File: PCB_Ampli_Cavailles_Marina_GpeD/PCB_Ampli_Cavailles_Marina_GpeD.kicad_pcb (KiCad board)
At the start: 2 copper layers, 52 parts, among them J2 Conn_01x02, J3 Conn_01x03, Q1 2N2907, Q10 TIP32, Q11 BD138, Q12 TIP31, Q13 2N2222, Q2 2N2907, Q3 2N2907, Q4 2N2222, Q5 2N2222, Q6 2N2907, Q7 2N2907, Q8 BD139, Q9 BD139, U1 Relay_1CT, U2 Jack_Mono

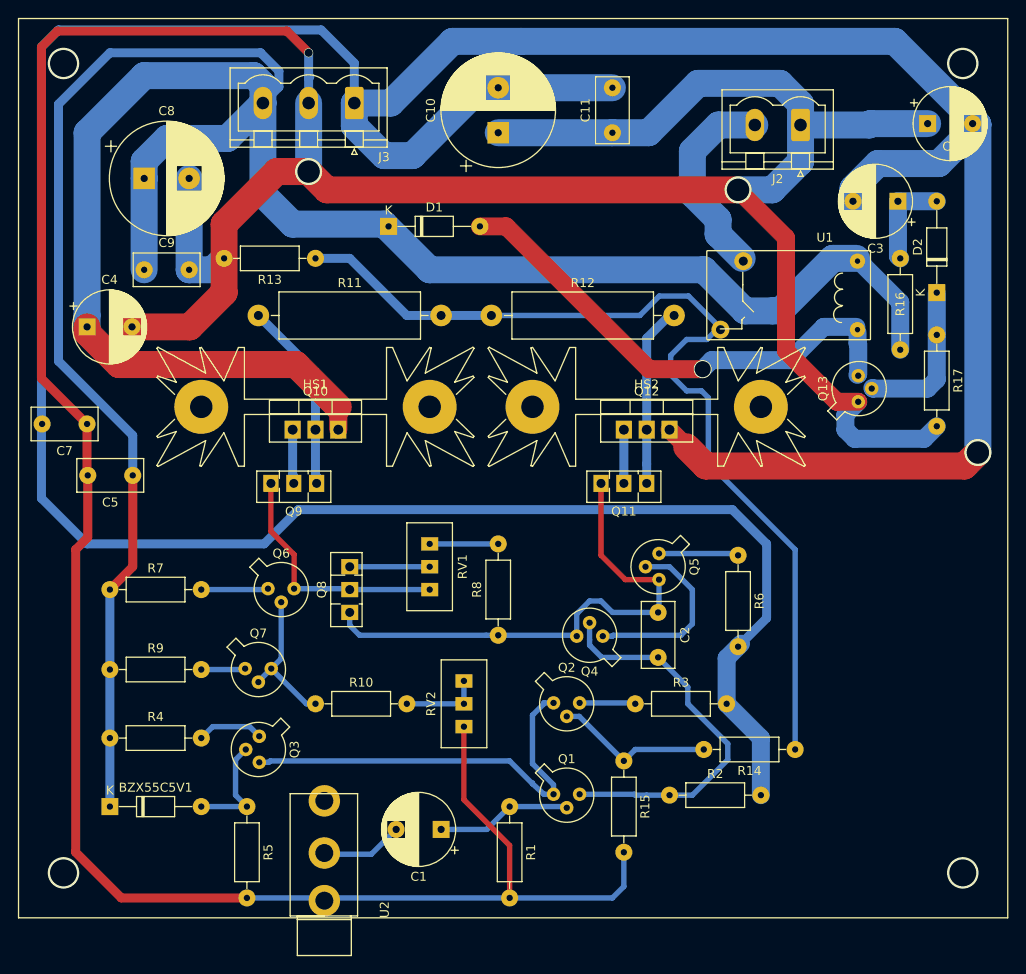
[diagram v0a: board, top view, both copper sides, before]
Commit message: Quatrième PCB (plaque de masse inclus)
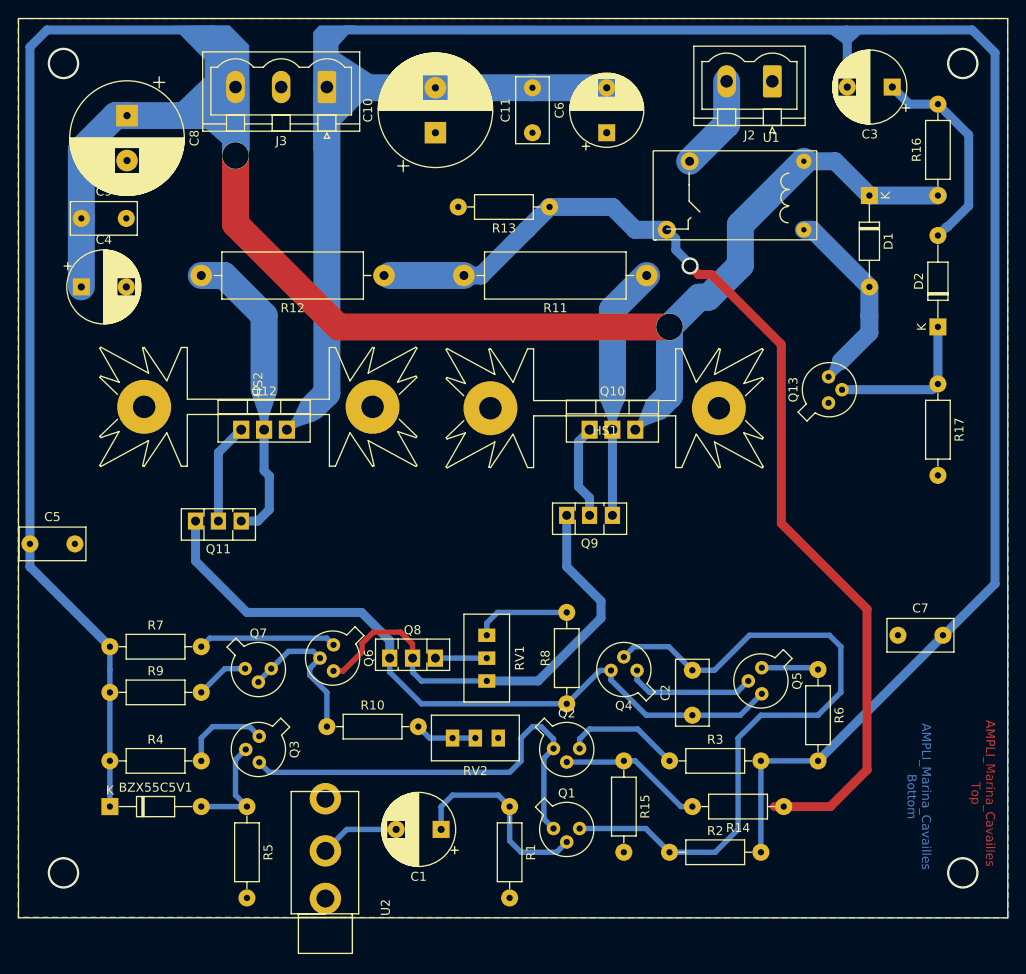
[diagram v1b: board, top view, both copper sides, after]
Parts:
- moved C7 93.2 mm to (123.2, 94.0), turned to 0 degrees
- moved D1 53.6 mm to (120.0, 45.1), turned to 270 degrees
- moved Q11 45.3 mm to (50.2, 81.3)
- moved R11 43.4 mm to (95.2, 54.0), turned to 180 degrees
- moved HS2 43.2 mm to (52.1, 68.6)
- moved Q12 42.5 mm to (50.2, 71.1)
- moved C6 35.7 mm to (90.8, 38.1), turned to 90 degrees
- moved Q9 33.1 mm to (91.4, 80.6)
- moved Q10 33.0 mm to (88.9, 71.1)
- moved HS1 32.2 mm to (90.6, 68.7), turned to 180 degrees
- moved R13 26.7 mm to (84.5, 46.4)
- moved R16 17.6 mm to (127.6, 45.1)
- moved Q5 17.1 mm to (108.0, 97.8)
- moved R6 15.5 mm to (114.3, 97.8)
- moved C5 13.7 mm to (26.7, 83.8), turned to 0 degrees
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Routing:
- net GND: track 432.5 -> 0.91 mm, vias 3 -> 0
- net -12V: track 414.3 -> 266.6 mm, vias 1 -> 0
- net +12V: track 319.4 -> 276.8 mm, vias 0 -> 2
- net Net-(D1-Pad2): track 55.2 -> 21.8 mm, vias 1 -> 0
- net Net-(C2-Pad2): track 43.4 -> 76.2 mm
- net Net-(Q6-Pad3): track 27.9 -> 52.1 mm
- net Net-(C2-Pad1): track 59.1 -> 81.2 mm
- net Net-(Q11-Pad1): track 19.7 -> 34.3 mm
- net Net-(C3-Pad1): track 10.8 -> 23.4 mm
- net Net-(J2-Pad2): track 22.4 -> 10.6 mm
- net Net-(R11-Pad2): track 106.6 -> 117.1 mm, vias 0 -> 1
- net Net-(Q6-Pad1): track 7.46 -> 15.4 mm
- net Net-(C1-Pad1): track 15.1 -> 22.4 mm
- net Net-(Q10-Pad2): track 21.4 -> 28.2 mm
- net Net-(Q2-Pad3): track 6.23 -> 13.0 mm
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- added copper zone on B.Cu, net GND
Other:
- net class Default: via_dia 0.8 -> 1.9
- net class FeCl3: clearance 0.2 -> 0.3; via_dia 0.8 -> 1.9
- rule via_min_size: 0.4 -> 1.9
- board text added: "AMPLI_Marina_Cavailles Bottom"
- board text added: "AMPLI_Marina_Cavailles Top"
- board text added: "EC DIFF"
- board text added: "PUISSANCE"
- board text removed: "DIFF EC"
- board text removed: "Puissance"
